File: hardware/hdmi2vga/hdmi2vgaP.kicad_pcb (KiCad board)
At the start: 2 copper layers, 44.7 x 31.4 mm, 27 parts, among them J1 HDMI, J2 VGA, J3 Composite

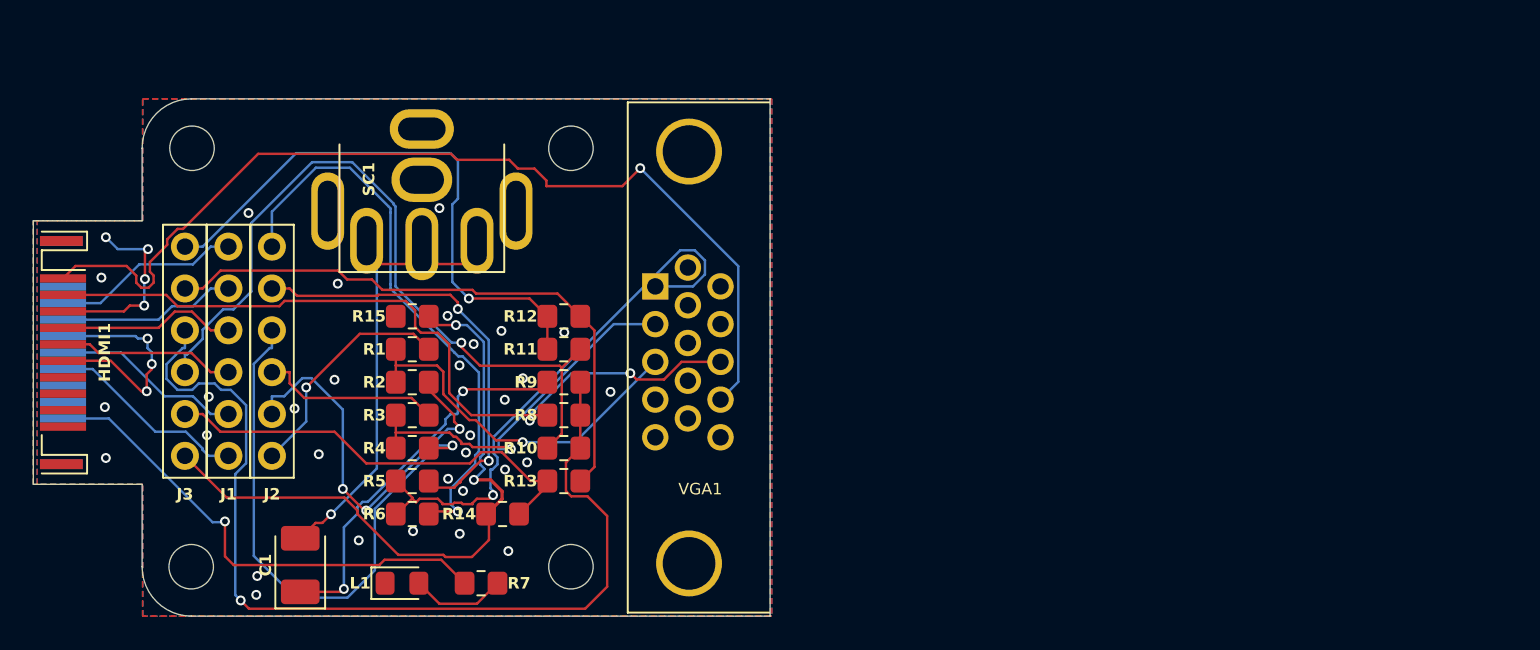
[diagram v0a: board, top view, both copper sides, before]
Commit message: Minor updates
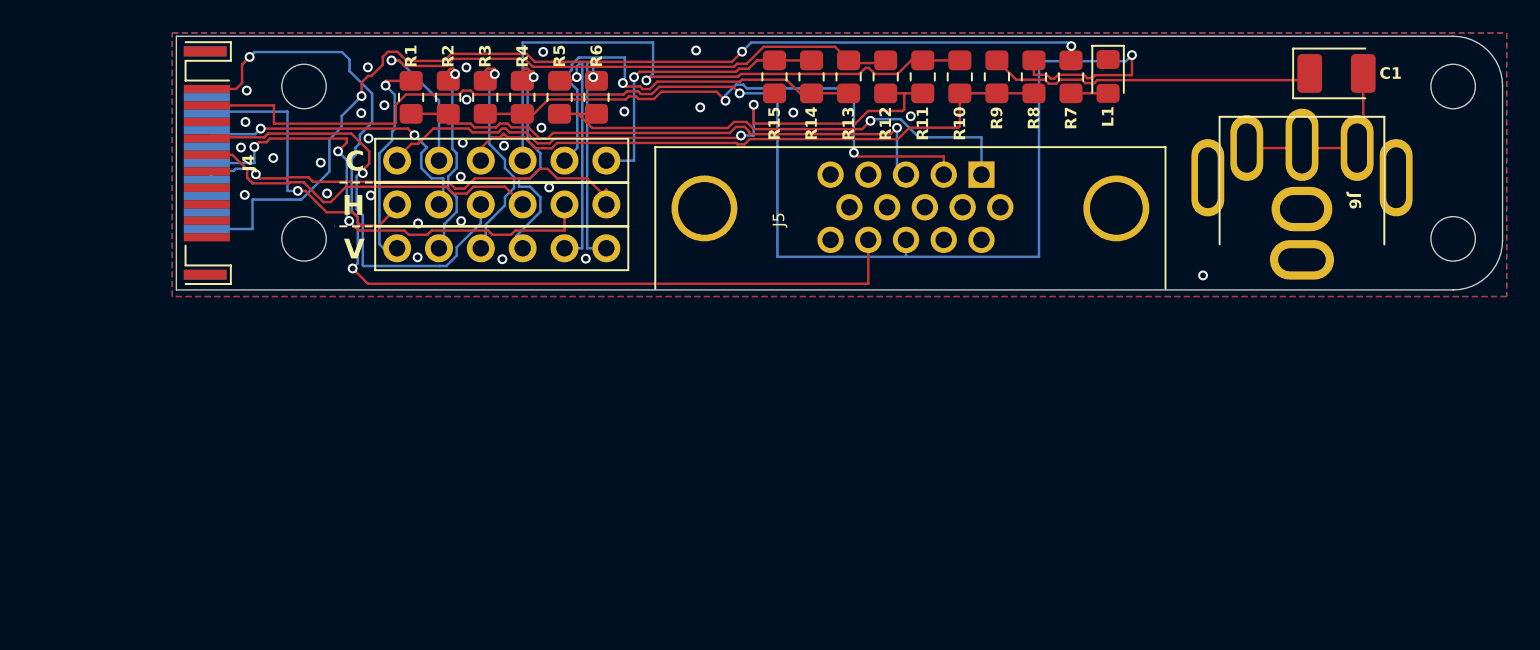
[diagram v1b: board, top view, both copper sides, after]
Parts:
- removed HDMI1: HDMI, FRANK:HDMI (male)
- removed SC1: VIDEO (Soft Composite), FRANK:RCA
- removed VGA1: VGA, FRANK:D-SUB (15 pin, female)
- added J4: HDMI, FRANK:HDMI (male), F.Cu at (140.1, 65.9)
- added J5: VGA, FRANK:D-SUB (15 pin, female), F.Cu at (187.1, 66.6)
- added J6: VIDEO (Soft Composite), FRANK:RCA, F.Cu at (206.6, 68.1)
- moved H3 82.0 mm to (215.8, 61.2)
- moved H4 76.7 mm to (215.8, 70.5)
- moved C1 69.6 mm to (208.7, 60.5), turned to 0 degrees
- moved L1 52.8 mm to (194.8, 60.6), turned to -90 degrees
- moved R7 47.2 mm to (192.6, 60.7), turned to -90 degrees
- moved R8 35.2 mm to (190.3, 60.7), turned to -90 degrees
- moved R10 32.9 mm to (185.8, 60.7), turned to -90 degrees
- moved R14 32.5 mm to (176.8, 60.7), turned to -90 degrees
- moved R9 32.2 mm to (188.1, 60.7), turned to 90 degrees
- moved J3 31.2 mm to (164.3, 65.8), turned to -90 degrees
- moved R13 30.0 mm to (179.1, 60.7), turned to 90 degrees
- moved R6 27.7 mm to (163.8, 61.9), turned to -90 degrees
- moved J1 27.6 mm to (164.3, 68.4), turned to -90 degrees
- moved R11 27.3 mm to (183.6, 60.7), turned to 90 degrees
- moved R15 26.4 mm to (174.6, 60.7), turned to 90 degrees
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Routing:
- net /HDMI/D2N: track 48.9 -> 90.7 mm
- net /HDMI/VBUS: track 30.1 -> 61.5 mm, vias 1 -> 3
- net GND: track 25.9 -> 0.00 mm, vias 38 -> 31
- net /Soft Composite/D0P: track 59.0 -> 36.9 mm, vias 1 -> 0
- net /Soft Composite/CLKN: track 39.8 -> 17.9 mm, vias 2 -> 1
- net Net-(J2-Pin_6): track 34.7 -> 13.7 mm
- net Net-(J2-Pin_4): track 34.9 -> 14.5 mm
- net /HDMI/CLKP: track 11.6 -> 30.5 mm, vias 0 -> 3
- net /Soft Composite/CVBS: track 29.0 -> 11.4 mm, vias 1 -> 0
- net /HDMI/D0P: track 10.9 -> 27.5 mm, vias 0 -> 1
- net /HDMI/CLKN: track 12.3 -> 27.2 mm, vias 0 -> 1
- net Net-(J2-Pin_5): track 26.6 -> 14.5 mm, vias 2 -> 1
- net Net-(J2-Pin_2): track 24.3 -> 12.5 mm, vias 3 -> 1
- net /VGA/VGA_BH: track 22.5 -> 34.2 mm
- net /HDMI/D0N: track 10.7 -> 21.9 mm
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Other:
- board size 44.7 x 31.4 mm -> 80.5 x 15.4 mm
- board text added: "2.02"
- board text added: "C"
- board text added: "H"
- board text added: "V"
- board text removed: "HW 2.01"
